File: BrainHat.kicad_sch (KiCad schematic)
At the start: 31 parts, among them J1 Electrodes, J2 Output, J3 Power, J4 Status, U1 AD8232, U2 TS5A3159ADBVR

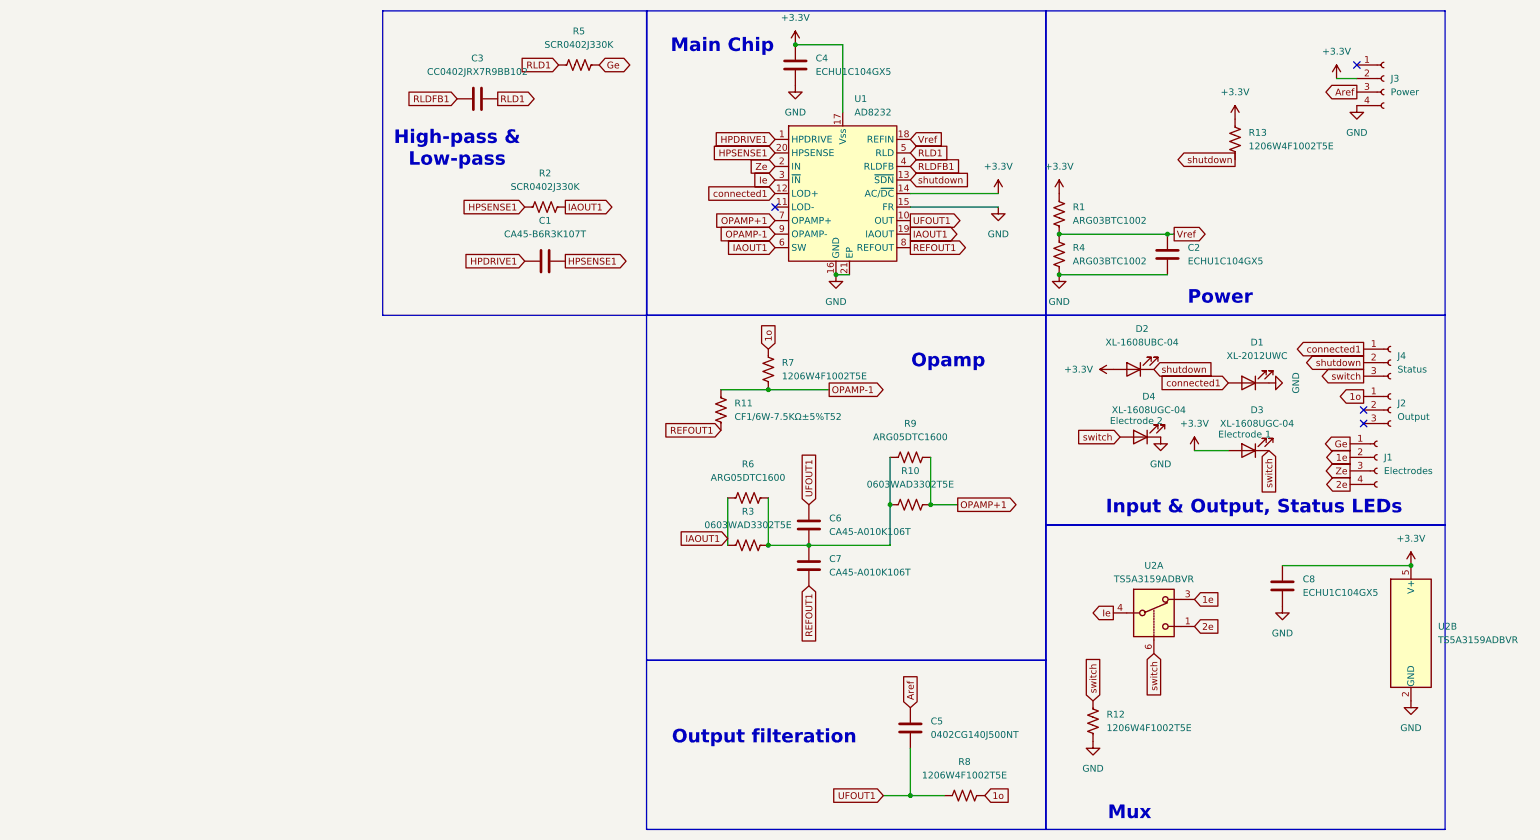
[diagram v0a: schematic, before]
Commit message: Started work on version 2
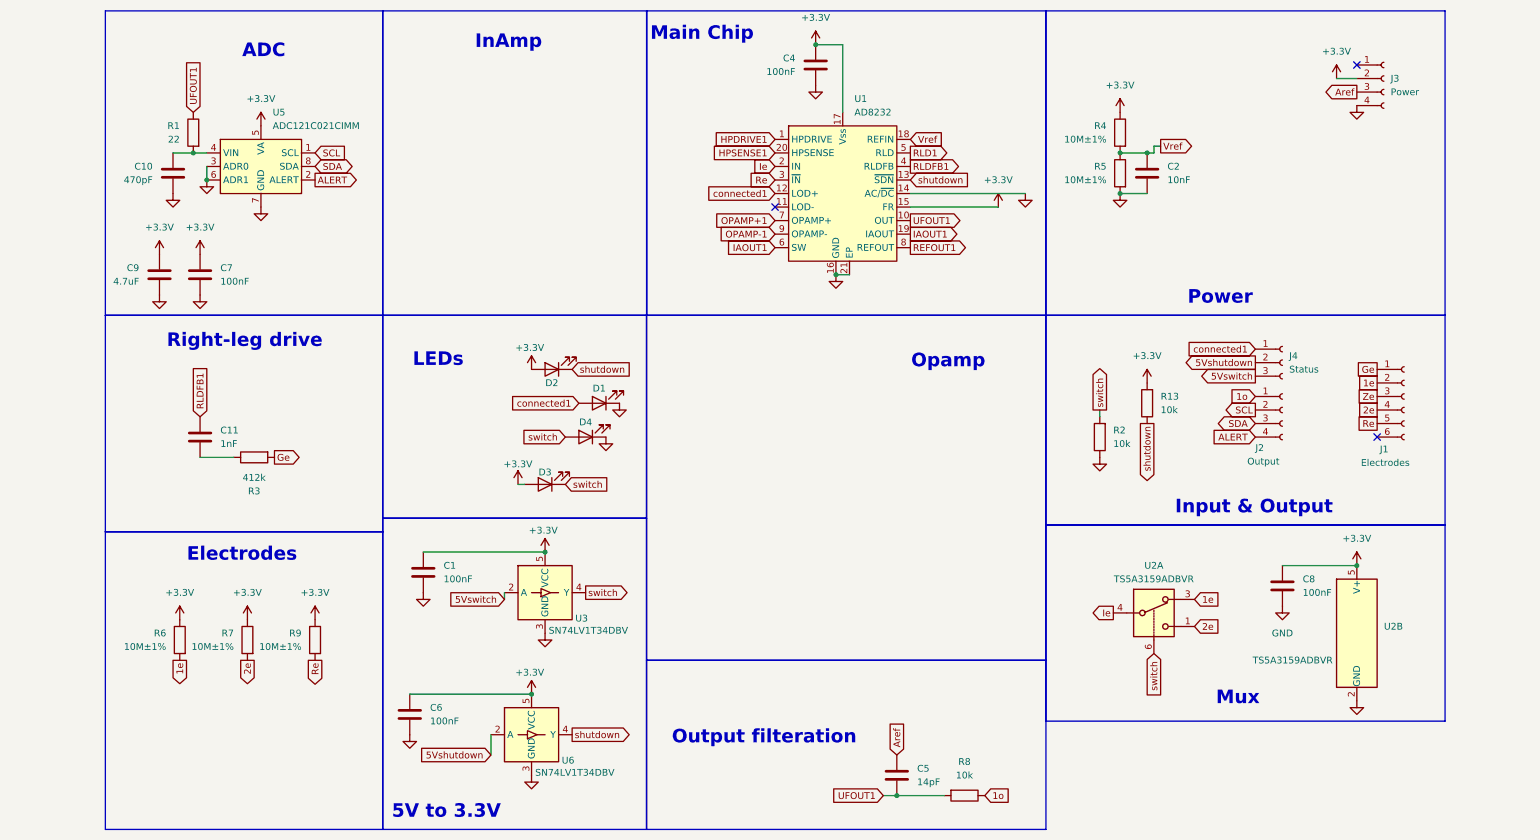
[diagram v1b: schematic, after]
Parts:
- removed C3: CC0402JRX7R9BB102, Capacitor_SMD:C_0402_1005Metric, symbol Device:C
- removed J1: Electrodes, Connector_PinSocket_2.54mm:PinSocket_1x04_P2.54mm_Vertical, symbol Connector:Conn_01x04_Socket
- removed J2: Output, Connector_PinSocket_2.54mm:PinSocket_1x03_P2.54mm_Vertical, symbol Connector:Conn_01x03_Socket
- removed R1, R4: ARG03BTC1002, Resistor_SMD:R_0603_1608Metric, symbol Device:R_US
- removed R10, R3: 0603WAD3302T5E, Resistor_SMD:R_0603_1608Metric, symbol Device:R_US
- removed R11: CF1/6W-7.5KΩ±5%T52, Personal:R_Axial_DIN0207_L6.3mm_D2.5mm_P5.08mm_Horizontal, symbol Device:R_US
- removed R12, R7, R8: 1206W4F1002T5E, Resistor_SMD:R_1206_3216Metric, symbol Device:R_US
- removed R2, R5: SCR0402J330K, Resistor_SMD:R_0402_1005Metric, symbol Device:R_US
- removed R6, R9: ARG05DTC1600, Resistor_SMD:R_0805_2012Metric, symbol Device:R_US
- added C10: 470pF, Capacitor_THT:C_Disc_D5.0mm_W2.5mm_P2.50mm, symbol Device:C
- added C11: 1nF, Capacitor_THT:C_Disc_D6.0mm_W4.4mm_P5.00mm, symbol Device:C
- added C9: 4.7uF, Capacitor_SMD:C_Elec_4x5.4, symbol Device:C
- added J1: Electrodes, Connector_PinHeader_2.54mm:PinHeader_1x06_P2.54mm_Vertical, symbol Connector:Conn_01x06_Socket
- added J2: Output, Connector_PinSocket_2.54mm:PinSocket_1x04_P2.54mm_Vertical, symbol Connector:Conn_01x04_Socket
- added R1: 22, Resistor_SMD:R_0402_1005Metric, symbol Device:R
- added R2, R8: 10k, Resistor_SMD:R_1206_3216Metric, symbol Device:R
- added R3: 412k, Resistor_SMD:R_2010_5025Metric, symbol Device:R
- added R4, R5, R6, R7, R9: 10M±1%, Resistor_THT:R_Axial_DIN0309_L9.0mm_D3.2mm_P15.24mm_Horizontal, symbol Device:R
- added U3, U6: SN74LV1T34DBV, Package_TO_SOT_SMD:SOT-23-5, symbol Logic_LevelTranslator:SN74LV1T34DBV
- added U5: ADC121C021CIMM, Package_SO:MSOP-8_3x3mm_P0.65mm, symbol Analog_ADC:ADC121C021CIMM
- C1: value CA45-B6R3K107T -> 100nF; footprint Capacitor_Tantalum_SMD:CP_EIA-3528-21_Kemet-B -> Capacitor_SMD:C_1210_3225Metric; LCSC Part # (none) -> C569766
- C2: value ECHU1C104GX5 -> 10nF; footprint Capacitor_SMD:C_1210_3225Metric -> Capacitor_THT:C_Disc_D12.0mm_W4.4mm_P7.75mm; LCSC Part # (none) -> C2896242
- C4, C8: value ECHU1C104GX5 -> 100nF; LCSC Part # (none) -> C569766
- C5: value 0402CG140J500NT -> 14pF; LCSC Part # (none) -> C3037644
- C6, C7: value CA45-A010K106T -> 100nF; footprint Capacitor_Tantalum_SMD:CP_EIA-3216-12_Kemet-S -> Capacitor_SMD:C_1210_3225Metric; LCSC Part # (none) -> C569766
- D1: LCSC Part # (none) -> C965818
- D2: LCSC Part # (none) -> C965807
- D3, D4: LCSC Part # (none) -> C965804
- J3: LCSC Part # (none) -> C5116530
- J4: LCSC Part # (none) -> C5116529
- R13: value 1206W4F1002T5E -> 10k; symbol Device:R_US -> Device:R; LCSC Part # (none) -> C17902
- U1: LCSC Part # (none) -> C43216
- U2: LCSC Part # (none) -> C128405
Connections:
- net +3.3V: now also C1.1, C6.1, C7.1, U1.15 (FR), C9.1, R4.1, R6.1, R7.1, R9.1, U3.5 (VCC), U5.5 (VA), U6.5 (VCC); no longer U1.14 (AC/~{DC})
- net 1e: now also J1.2 (Pin_2), R6.2
- net 1o: now also J2.1 (Pin_1), R8.1
- net 2e: now also J1.4 (Pin_4), R7.2
- net GND: now also C1.2, C6.2, C7.2, U1.14 (AC/~{DC}), C10.2, C9.2, R2.1, R5.2, U3.3 (GND), U5.3 (ADR0), U5.6 (ADR1), U5.7 (GND), U6.3 (GND); no longer U1.15 (FR)
- net Ge: now also J1.1 (Pin_1), R3.2
- net HPDRIVE1: no longer C1.1
- net HPSENSE1: no longer C1.2
- net Ie: now also U1.2 (IN); no longer U1.3 (~{IN})
- net REFOUT1: no longer C7.1
- net RLDFB1: now also C11.1
- net UFOUT1: now also R1.1, R8.2; no longer C6.2
- net Vref: now also R4.2, R5.1
- net Ze: now also J1.3 (Pin_3); no longer U1.2 (IN)
- net shutdown: now also U6.4 (Y); no longer J4.2 (Pin_2)
- net switch: now also R2.2, U3.4 (Y); no longer J4.3 (Pin_3)
- new net: C11.2, R3.1
- new net: C10.1, R1.2, U5.4 (VIN)
- new net 5Vshutdown: J4.2 (Pin_2), U6.2 (A)
- new net 5Vswitch: J4.3 (Pin_3), U3.2 (A)
- new net ALERT: J2.4 (Pin_4), U5.2 (ALERT)
- new net Re: J1.5 (Pin_5), R9.2, U1.3 (~{IN})
- new net SCL: J2.2 (Pin_2), U5.1 (SCL)
- new net SDA: J2.3 (Pin_3), U5.8 (SDA)
- no-connect marks 4 -> 3
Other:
- note added: "5V to 3.3V"
- note added: "ADC"
- note added: "Electrodes"
- note added: "InAmp"
- note added: "Input & Output"
- note added: "LEDs"
- note added: "Right-leg drive"
- note removed: "High-pass & Low-pass"
- note removed: "Input & Output, Status LEDs"
- company: (none) -> BrainHat, LLC
- title: (none) -> Main BrainHat Bio-Potential Amplifier
- moved on the sheet: C4, C5, D1, D2, D3, D4, J4, U2B

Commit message: YAAAA
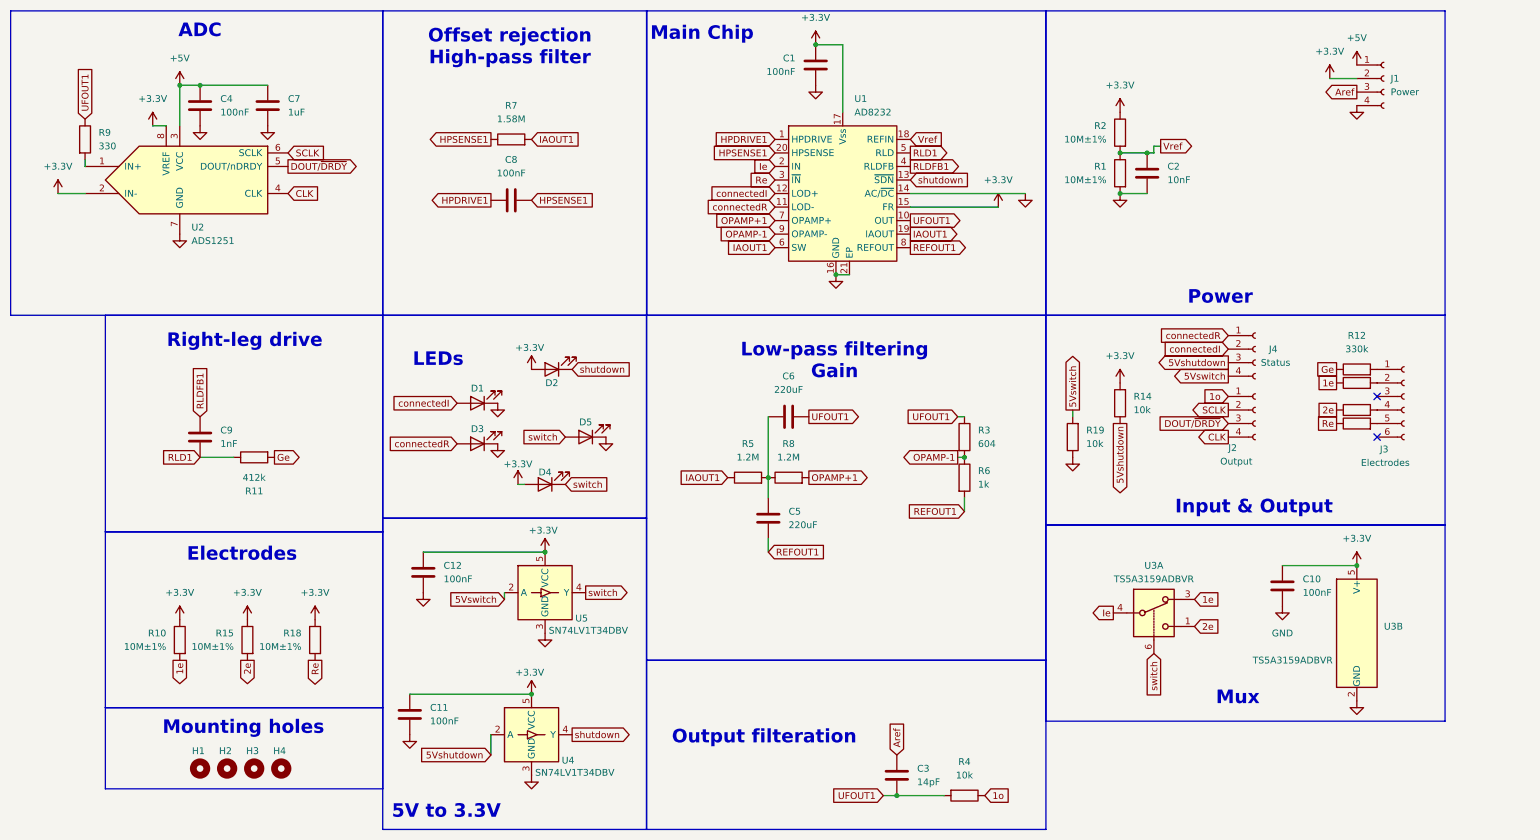
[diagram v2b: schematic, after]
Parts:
- removed C10: 470pF, Capacitor_THT:C_Disc_D5.0mm_W2.5mm_P2.50mm, symbol Device:C
- removed C9: 4.7uF, Capacitor_SMD:C_Elec_4x5.4, symbol Device:C
- removed J4: Status, Connector_PinSocket_2.54mm:PinSocket_1x03_P2.54mm_Vertical, symbol Connector:Conn_01x03_Socket
- removed R1: 22, Resistor_SMD:R_0402_1005Metric, symbol Device:R
- removed U5: ADC121C021CIMM, Package_SO:MSOP-8_3x3mm_P0.65mm, symbol Analog_ADC:ADC121C021CIMM
- added C4, C8: 100nF, Capacitor_SMD:C_1210_3225Metric, symbol Device:C
- added C5, C6: 220uF, Capacitor_SMD:C_Elec_6.3x5.4, symbol Device:C
- added D3: XL-2012UWC, LED_SMD:LED_0805_2012Metric, symbol Device:LED
- added H1, H2, H3, H4: MountingHole, MountingHole:MountingHole_2.2mm_M2, symbol Mechanical:MountingHole
- added J4: Status, Connector_PinSocket_2.54mm:PinSocket_1x04_P2.54mm_Vertical, symbol Connector:Conn_01x04_Socket
- added R12, R13, R16, R17: 330k, Resistor_SMD:R_0402_1005Metric, symbol Device:R
- added R3: 604, Resistor_SMD:R_0402_1005Metric, symbol Device:R
- added R5, R8: 1.2M, Resistor_SMD:R_0402_1005Metric, symbol Device:R
- added R6: 1k, Resistor_SMD:R_0402_1005Metric, symbol Device:R
- added R7: 1.58M, Resistor_SMD:R_0402_1005Metric, symbol Device:R
- added R9: 330, Resistor_SMD:R_0402_1005Metric, symbol Device:R
- added U2: ADS1251, Package_SO:MSOP-8_3x3mm_P0.65mm, symbol Analog_ADC:ADS1251
- C7: value 100nF -> 1uF; footprint Capacitor_SMD:C_1210_3225Metric -> Capacitor_THT:C_Disc_D5.1mm_W3.2mm_P5.00mm; LCSC Part # C569766 -> C2839237
- renumbered C4 to C1, C8 to C10, C6 to C11, C1 to C12, C5 to C3, C11 to C9, D3 to D4, D4 to D5, J3 to J1, J1 to J3, R5 to R1, R6 to R10, R3 to R11, R13 to R14, R7 to R15, R9 to R18, R2 to R19, R4 to R2, R8 to R4, U2 to U3, U6 to U4, U3 to U5
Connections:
- net +3.3V: now also U2.2 (IN-), U2.8 (VREF); no longer C7.1
- net 1e: now also R13.1; no longer J3.2 (Pin_2)
- net 2e: now also R16.1; no longer J3.4 (Pin_4)
- net 5Vshutdown: now also R14.1, J4.3 (Pin_3)
- net 5Vswitch: now also R19.2, J4.4 (Pin_4)
- net GND: now also C4.2, D3.1 (K), U2.7 (GND)
- net Ge: now also R12.1; no longer J3.1 (Pin_1)
- net HPDRIVE1: now also C8.1
- net HPSENSE1: now also C8.2, R7.1
- net IAOUT1: now also R5.1, R7.2
- net OPAMP+1: now also R8.2
- net OPAMP-1: now also R3.2, R6.1
- net REFOUT1: now also C5.1, R6.2
- net RLD1: now also C9.2, R11.1
- net Re: now also R17.1; no longer J3.5 (Pin_5)
- net UFOUT1: now also C6.2, R3.1, R9.1
- net shutdown: no longer R14.1
- net switch: no longer R19.2
- net connectedR: now reaches U1.11 (LOD-)
- net connectedR: now also D3.2 (A), J4.1 (Pin_1)
- net +5V: now reaches J1.1 (Pin_1)
- net +5V: now also C7.1, C4.1, U2.3 (VCC)
- net ALERT renamed CLK
- net CLK: now also U2.4 (CLK)
- net SCL renamed SCLK
- net SCLK: now also U2.6 (SCLK)
- net SDA renamed DOUT/~{DRDY}
- net DOUT/~{DRDY}: now also U2.5 (DOUT/nDRDY)
- net Ze: no longer names the net of J3.3 (Pin_3)
- net connected1 renamed connectedI
- net connectedI: now also J4.2 (Pin_2)
- new net: R9.2, U2.1 (IN+)
- new net: C5.2, C6.1, R5.2, R8.1
- new net: J3.2 (Pin_2), R13.2
- new net: J3.1 (Pin_1), R12.2
- new net: J3.4 (Pin_4), R16.2
- new net: J3.5 (Pin_5), R17.2
- no-connect marks 3 -> 2
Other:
- note added: "Low-pass filtering Gain"
- note added: "Mounting holes"
- note added: "Offset rejection High-pass filter"
- note removed: "InAmp"
- note removed: "Opamp"
- moved on the sheet: D1, J2, R14, R19

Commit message: Changes
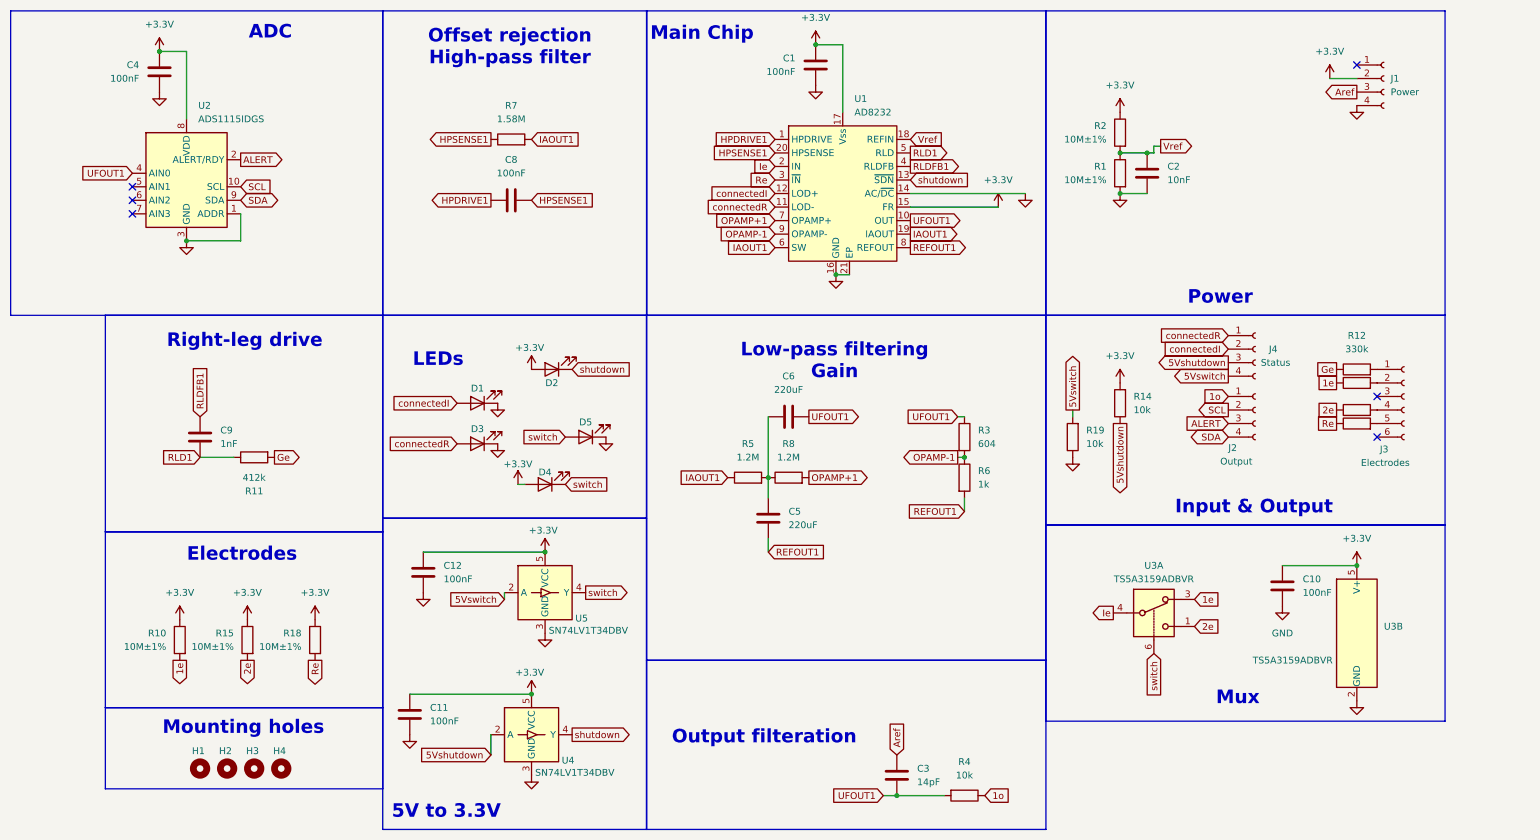
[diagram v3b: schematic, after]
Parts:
- removed C7: 1uF, Capacitor_THT:C_Disc_D5.1mm_W3.2mm_P5.00mm, symbol Device:C
- removed R9: 330, Resistor_SMD:R_0402_1005Metric, symbol Device:R
- removed U2: ADS1251, Package_SO:MSOP-8_3x3mm_P0.65mm, symbol Analog_ADC:ADS1251
- added U2: ADS1115IDGS, Package_SO:TSSOP-10_3x3mm_P0.5mm, symbol Analog_ADC:ADS1115IDGS
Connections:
- net +3.3V: now also C4.1, U2.8 (VDD)
- net GND: now also U2.1 (ADDR), U2.3 (GND)
- net UFOUT1: now also U2.4 (AIN0)
- net +5V: no longer names the net of J1.1 (Pin_1)
- net +5V: no longer C4.1
- net CLK renamed SDA
- net SDA: now also U2.9 (SDA)
- net DOUT/~{DRDY} renamed ALERT
- net ALERT: now also U2.2 (ALERT/RDY)
- net SCLK renamed SCL
- net SCL: now also U2.10 (SCL)
- no-connect marks 2 -> 6
